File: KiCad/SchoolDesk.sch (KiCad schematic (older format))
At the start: 15 parts, among them J1 Conn_1x5, J2 DIN-5_180degree, J3 Conn_1x1, J4 Conn_01x14_Female, J5 Conn_01x14_Female, J6 Conn_1x5

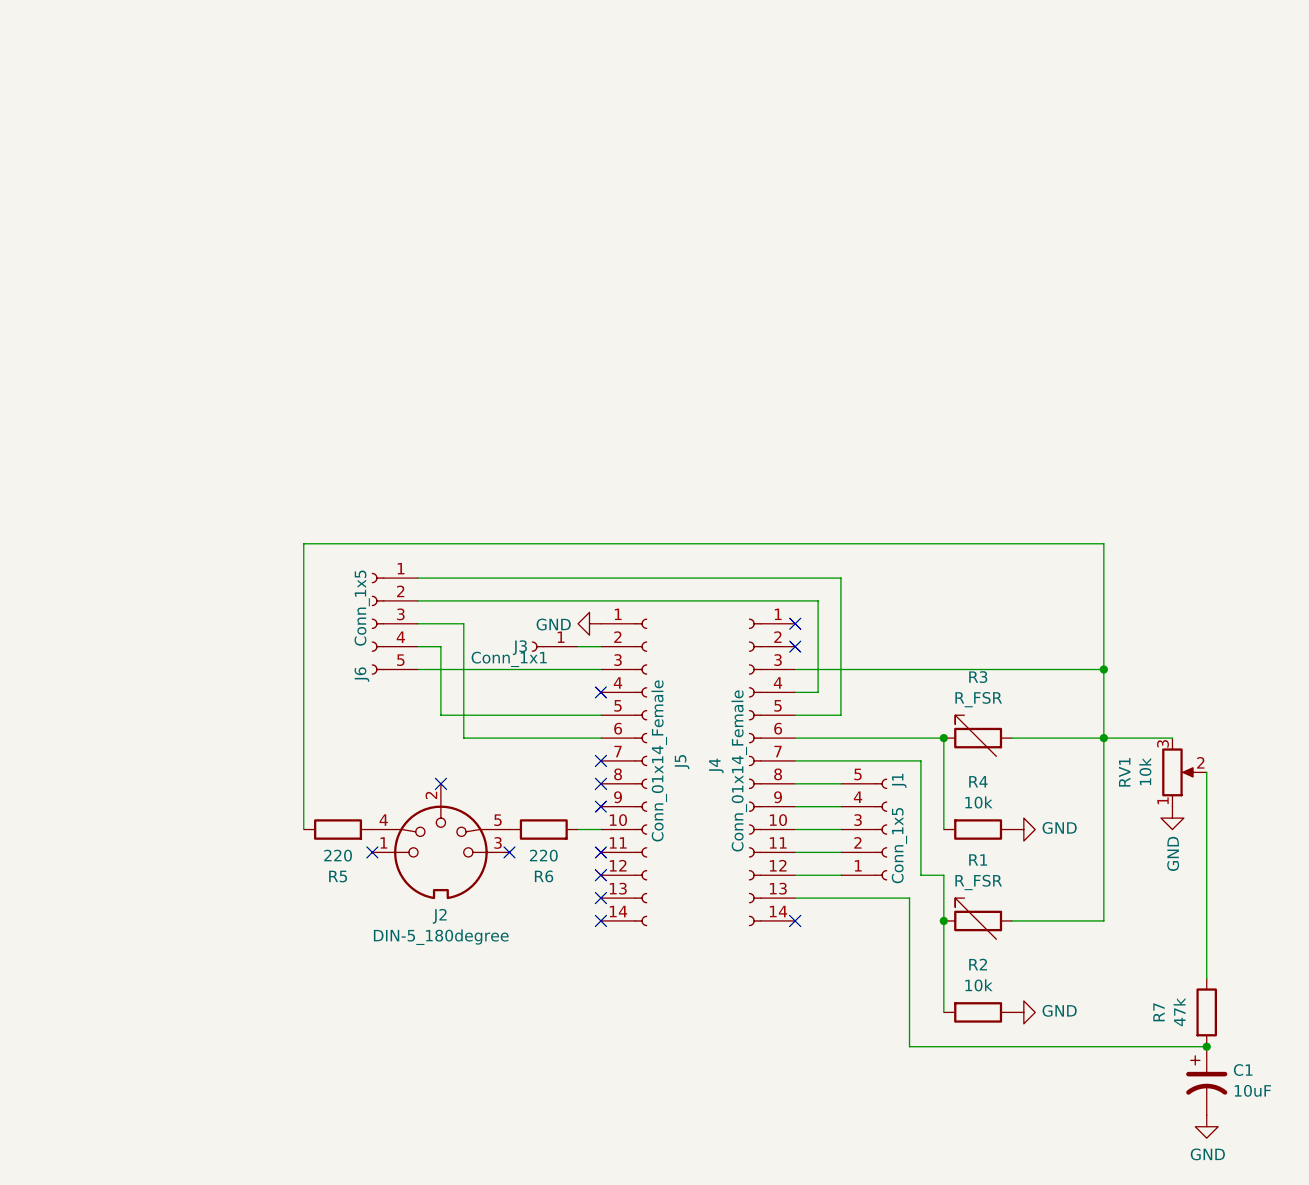
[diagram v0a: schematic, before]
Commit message: First (untested) commit including PCB files.
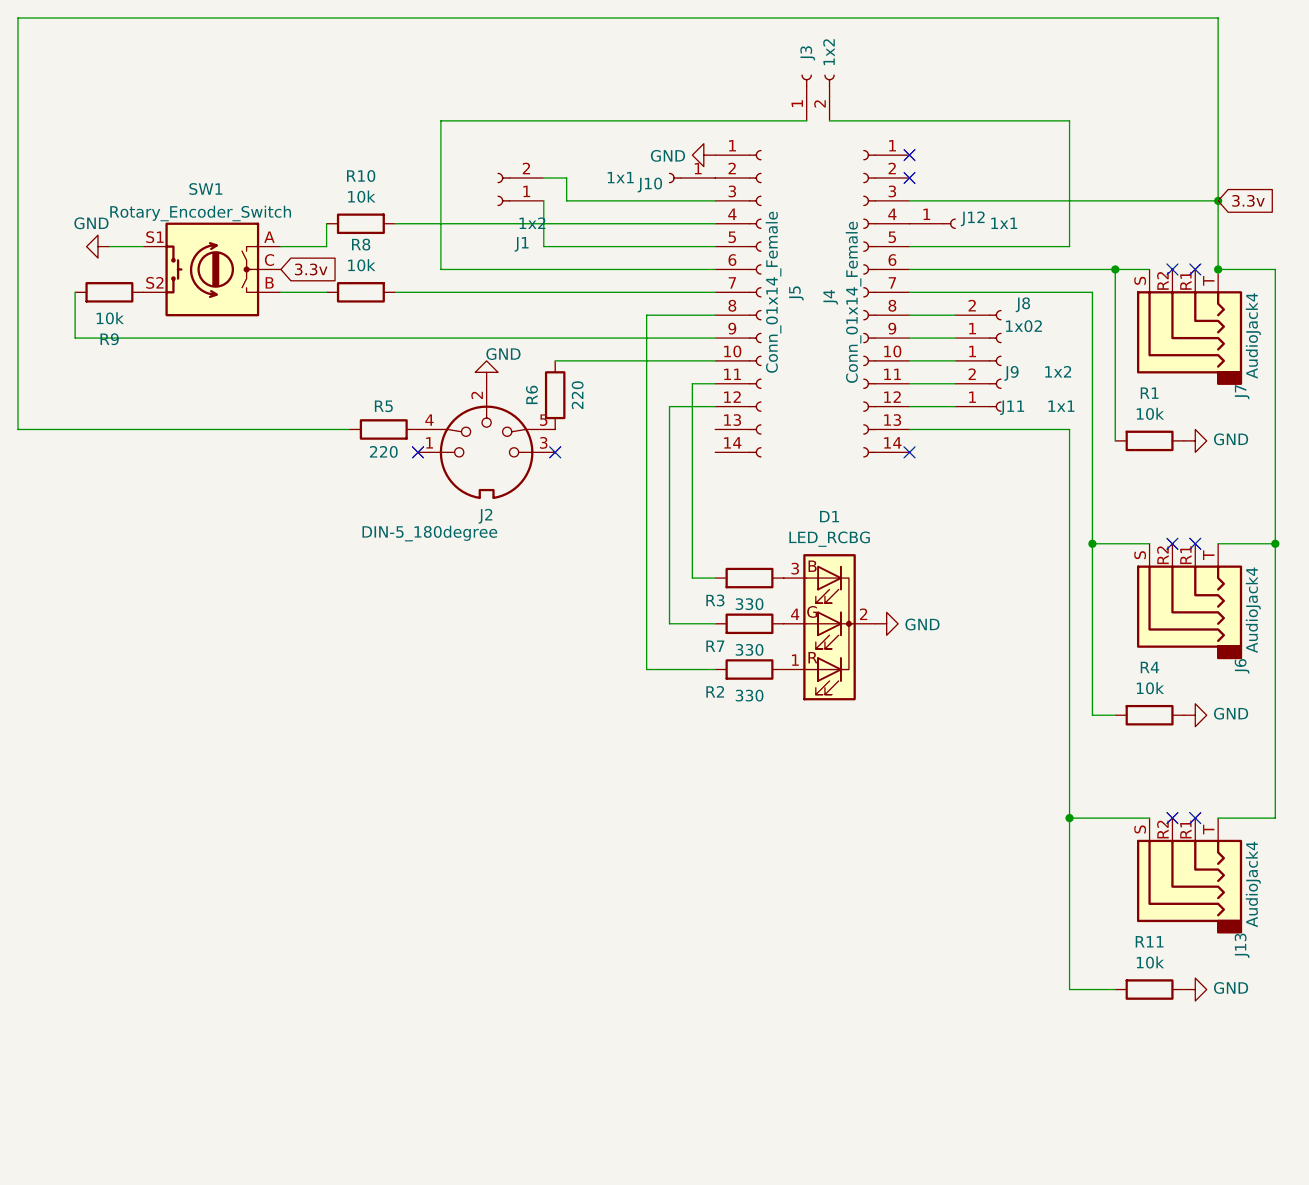
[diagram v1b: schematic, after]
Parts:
- removed C1: 10uF, C_SMD_3D:C_0805_2012Metric, symbol Device:CP1
- removed J1, J6: Conn_1x5, Pin_Headers:Pin_Header_Straight_1x05_Pitch2.00mm, symbol Connector:Conn_01x05_Female
- removed J3: Conn_1x1, P_2.54_3D:PinHeader_1x01_P2.54mm_Vertical, symbol Connector:Conn_01x01_Female
- removed R1, R3: R_FSR, Connectors:PJ320E_3.5mm_Jack, symbol Device:R_Variable
- removed RV1: 10k, Potentiometers:Potentiometer_Alps_RK09K_Vertical, symbol Device:R_POT
- added D1: LED_RCBG, LED_THT_3D:LED_D5.0mm-4_RGB, symbol Device:LED_RCBG
- added J1, J3, J9: 1x2, Pin_Headers:Pin_Header_Straight_1x02_Pitch2.00mm, symbol Connector:Conn_01x02_Female
- added J10, J11, J12: 1x1, Pin_Headers:Pin_Header_Straight_1x01_Pitch2.00mm, symbol Connector:Conn_01x01_Female
- added J13, J6, J7: AudioJack4, Conn_Aud_3D:Jack_3.5mm_PJ320D_Horizontal, symbol Connector:AudioJack4
- added J8: 1x02, Pin_Headers:Pin_Header_Straight_1x02_Pitch2.00mm, symbol Connector:Conn_01x02_Female
- added R1, R11: 10k, Resistors_ThroughHole:R_Axial_DIN0207_L6.3mm_D2.5mm_P2.54mm_Vertical, symbol Device:R
- added R10, R8, R9: 10k, R_SMD_3D:R_0805_2012Metric, symbol Device:R
- added R3: 330, R_SMD_3D:R_0805_2012Metric, symbol Device:R
- added SW1: Rotary_Encoder_Switch, digikey-footprints:Rotary_Encoder_Switched_PEC11R, symbol Device:Rotary_Encoder_Switch
- R2: value 10k -> 330; footprint Resistors_ThroughHole:R_Axial_DIN0207_L6.3mm_D2.5mm_P2.54mm_Vertical -> R_SMD_3D:R_0805_2012Metric
- R7: value 47k -> 330
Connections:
- net GND: now also J2.2, D1.2 (K), R1.1, R11.1, SW1.S1; no longer R2.1
- net at J4.7 (Pin_7): now also R4.2, J6.S; no longer R2.2
- net 3.3v: now reaches J4.3 (Pin_3), R5.1
- net 3.3v: now also J13.T, J6.T, J7.T, SW1.C
- net at J4.6 (Pin_6): now also J7.S, R1.2; no longer R4.2
- net at R7.1: now also D1.4 (GA)
- net at J4.13 (Pin_13): now also J13.S, R11.2; no longer R7.2
- net at J4.10 (Pin_10): now also J9.1 (Pin_1)
- net at J4.11 (Pin_11): now also J9.2 (Pin_2)
- net at J4.12 (Pin_12): now also J11.1 (Pin_1)
- net at J4.4 (Pin_4): now also J12.1 (Pin_1)
- net at J4.5 (Pin_5): now also J3.2 (Pin_2)
- net at J4.8 (Pin_8): now also J8.2 (Pin_2)
- net at J4.9 (Pin_9): now also J8.1 (Pin_1)
- net at J5.10 (Pin_10): now also R6.1; no longer R6.2
- net at J5.11 (Pin_11): now also R3.2
- net at J5.12 (Pin_12): now also R7.2
- net at J5.2 (Pin_2): now also J10.1 (Pin_1)
- net at J5.3 (Pin_3): now also J1.2 (Pin_2)
- net at J5.4 (Pin_4): now also R10.2
- net at J5.5 (Pin_5): now also J1.1 (Pin_1)
- net at J5.6 (Pin_6): now also J3.1 (Pin_1)
- net at J5.7 (Pin_7): now also R8.2
- net at J5.8 (Pin_8): now also R2.2
- net at J5.9 (Pin_9): now also R9.2
- net at J2.5: now also R6.2; no longer R6.1
- new net: R10.1, SW1.A
- new net: R8.1, SW1.B
- new net: R9.1, SW1.S2
- new net: D1.1 (RA), R2.1
- new net: D1.3 (BA), R3.1
- no-connect marks 14 -> 11
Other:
- moved on the sheet: J2, J4, J5, R4, R5, R6
